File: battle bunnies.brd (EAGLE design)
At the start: 113 x 33 mm, 48 parts, among them IC1 CP2104, Q1 mmbt2222, Q2 mmbt2222, Q3 DMG3415U, SW2 KMR2, U2 AP2112-3.3, U3 MCP73831T-2ACI/OT, U4 BMEx80, X2 ESP32_WROOM32_SKINNY, X4 20329

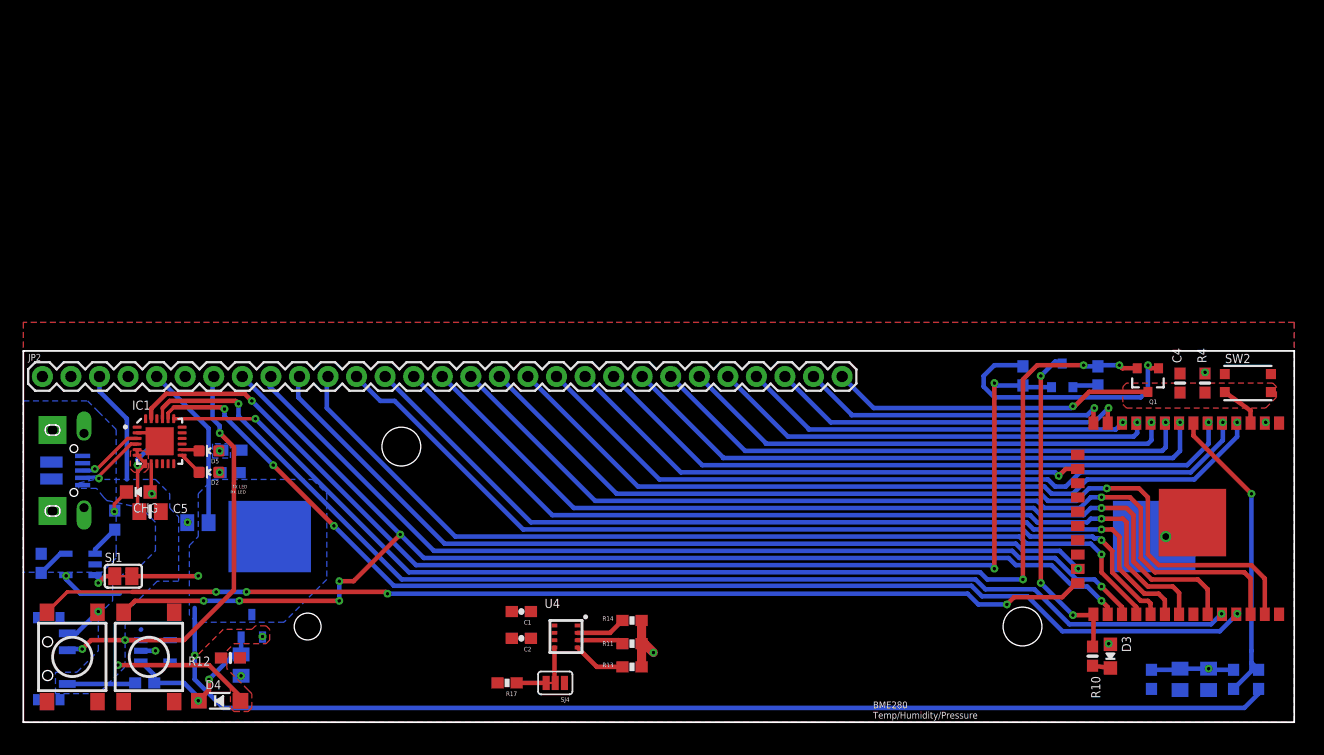
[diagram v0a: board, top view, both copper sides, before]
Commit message: Big changes - 'final' routing, light sensor, bme280 -> bme680
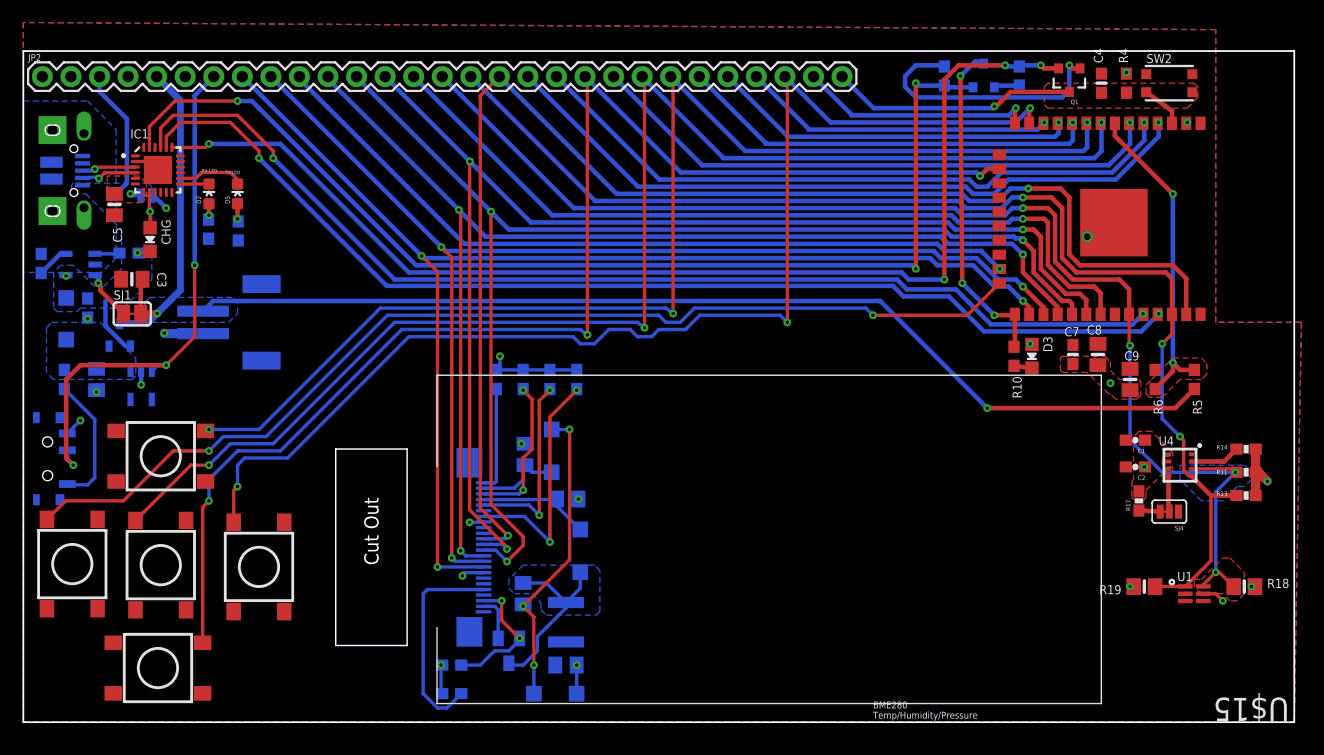
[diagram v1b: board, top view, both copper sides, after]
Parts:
- removed U$31: 18650, Warthog9-Batteries:KEYSTONE1042
- added BT1: LIPO-OUTLINE2000, SparkFun-Batteries:LIPO-2000
- added C10, C11, C12: 1µF, microbuilder:0805-NO@1
- added C13: 2.2µF, microbuilder:0805-NO@1
- added C14, C15, C16, C17, C18: 1uF, SparkFun-Capacitors:0603-CAP
- added D1, D6, D7: MBR0520LT, diode:SOD123
- added J1: (no value), SparkFun-Connectors:JST-2-SMD
- added L1: INDUCTOR-1812-68uH-220ma, SparkFun-Coils:1812
- added Q4: (no value), adafruit:SOT23
- added R16: 2.2, SparkFun-Resistors:0603-RES
- added R18, R19: 10K, microbuilder:0805-NO
- added S4, S5, S6: SWITCH-MOMENTARY-2SMD-4, SparkFun-Electromechanical:TACTILE_SWITCH_TALL
- added U$15: WAVSHARE-BUYDISPLAY-2.132.13-THROUGH, Warthog9-Screens:WAVSHARE-BUYDISPLAY-2.13-THM
- added U1: TSL2591, microbuilder:DFN6_TAOS
- C3, C5, C6, C8, C9: device microbuilder:0805-NO -> microbuilder:0805-NO@1
- C4, C7: device microbuilder:0603-NO -> microbuilder:0603-NO@1
- moved R17 58.5 mm to (99.2, 19.7), turned to 90 degrees
- moved C1 56.7 mm to (98.9, 25.1)
- moved C2 56.7 mm to (98.9, 22.7)
- moved R11 56.7 mm to (108.7, 22.2)
- moved R13 56.7 mm to (108.7, 20.2)
- moved R14 56.7 mm to (108.7, 24.3)
- moved SJ4 56.7 mm to (101.9, 18.7)
- moved U4 56.7 mm to (102.9, 22.9)
- moved D4 36.6 mm to (3.81, 35.9), flipped to the bottom, turned to 90 degrees
- moved R12 33.6 mm to (5.71, 36.8), flipped to the bottom, turned to 90 degrees
- moved C8 29.8 mm to (95.6, 32.7), flipped to the top
- moved C7 29.7 mm to (93.3, 32.7), flipped to the top
- moved C6 28.5 mm to (6.51, 30.5)
- moved Q3 28.4 mm to (8.57, 34.4)
- moved R7 27.9 mm to (3.65, 30.5), turned to 90 degrees
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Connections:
- new net GDR: Q4.1, U$15.2-GDR
- new net N$11: C12.1, D1.C, D6.A
- new net N$14: C12.2, D7.A, L1.1, Q4.3
- new net N$16: C15.1, U$15.18-VDD
- new net N$17: C16.1, U$15.20-VSH
- new net N$18: C17.1, U$15.22-VSL
- new net N$19: C18.1, U$15.24-VCOM
- new net N$20: C14.1, U$15.5-VGH
- new net RESE: Q4.2, R16.1, U$15.3-RESE
- new net VGH: C10.2, D7.C, U$15.21-PREVGH
- new net VGL: C11.2, D1.A, U$15.23-PREVGL
- net 3.3V: now also C13.1, L1.2, R18.2, R19.2, U$15.15-VDDIO, U$15.16-VCI, U1.5
- net A5_IO4: now also U$15.9-BUSY; no longer S2.B2
- net GND: now also C10.1, C11.1, C13.2, C14.2, C15.2, C16.2, C17.2, C18.2, D6.C, J1.1, R16.2, S4.A2, S5.A2, S6.A2, U$15.17-GND, U$15.8-BS1, U1.3; no longer U$31.NEG
- net IO13_A12: now also S2.B2
- net IO14_A6: now also S4.B2
- net IO16: now also U$15.10-RES#
- net IO17: now also U$15.11-D/C#
- net IO23: now also U$15.14-D1
- net IO32_A7: now also S6.B2
- net IO33_A9: now also S5.B2
- net MOSI: now also U$15.13-D0
- net SCK: now also U$15.12-CS#
- net SCL: now also R19.1, U1.1
- net SDA: now also R18.1, U1.6
- net VBAT: now also J1.2; no longer U$31.POS
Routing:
- net IO14_A6: track 32.4 -> 108.3 mm, vias 1 -> 3
- net IO13_A12: track 47.7 -> 117.9 mm, vias 1 -> 3
- net IO32_A7: track 53.8 -> 121.9 mm, vias 1 -> 3
- net IO33_A9: track 49.2 -> 109.7 mm, vias 1 -> 3
- net IO23: track 82.6 -> 120.4 mm, vias 1 -> 2
- net MOSI: track 80.5 -> 111.7 mm, vias 1 -> 3
- net SDA: track 85.2 -> 113.7 mm, vias 1 -> 4
- net SCK: track 81.1 -> 109.5 mm, vias 1 -> 3
- net N$11: track 0.00 -> 27.4 mm, vias 0 -> 3
- net IO17: track 83.7 -> 107.8 mm, vias 1 -> 3
- net IO16: track 85.5 -> 109.0 mm, vias 1 -> 3
- net N$16: track 0.00 -> 21.4 mm, vias 0 -> 2
- net SCL: track 88.1 -> 108.8 mm, vias 1 -> 3
- net N$20: track 0.00 -> 18.9 mm
- net N$17: track 0.00 -> 16.9 mm, vias 0 -> 2
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- added copper zone on layer 1, net 3.3V
- added copper zone on layer 1, net A13_I35
- added copper zone on layer 16, net N$14
- added copper zone on layer 16, net N$7
- added copper zone on layer 1, net SDA
- added copper zone on layer 16, net SDA
- removed copper zone on layer 16, net N$8
- removed copper zone on layer 1, net VBUS
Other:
- board size 113 x 33 mm -> 113 x 59.7 mm
